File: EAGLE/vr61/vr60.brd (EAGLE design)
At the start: 283 x 93 mm, 222 parts, among them IC1 MC74VHC1G50, IC2 REG1117, J6 MICROMOD-2222-C

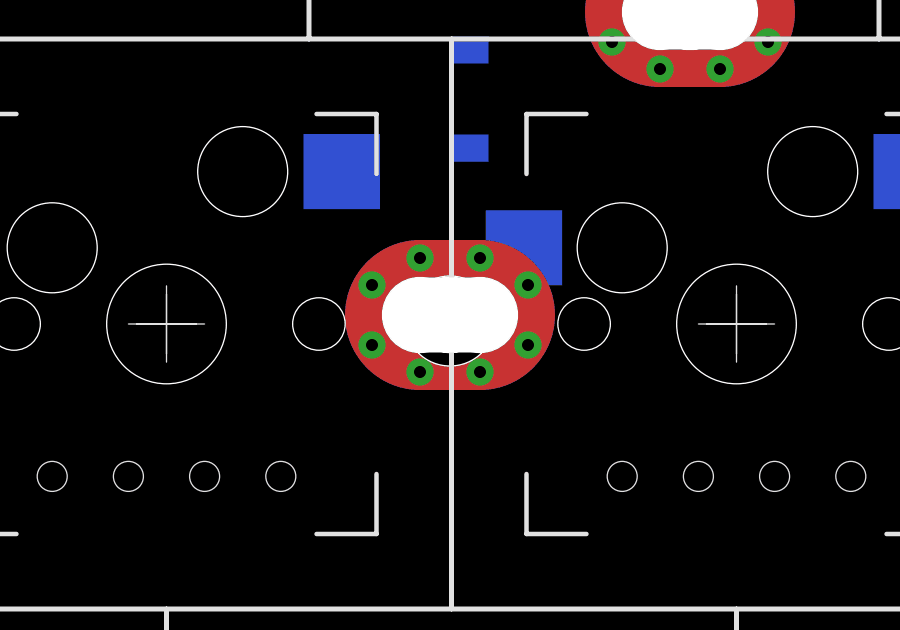
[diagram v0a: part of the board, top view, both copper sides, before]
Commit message: .
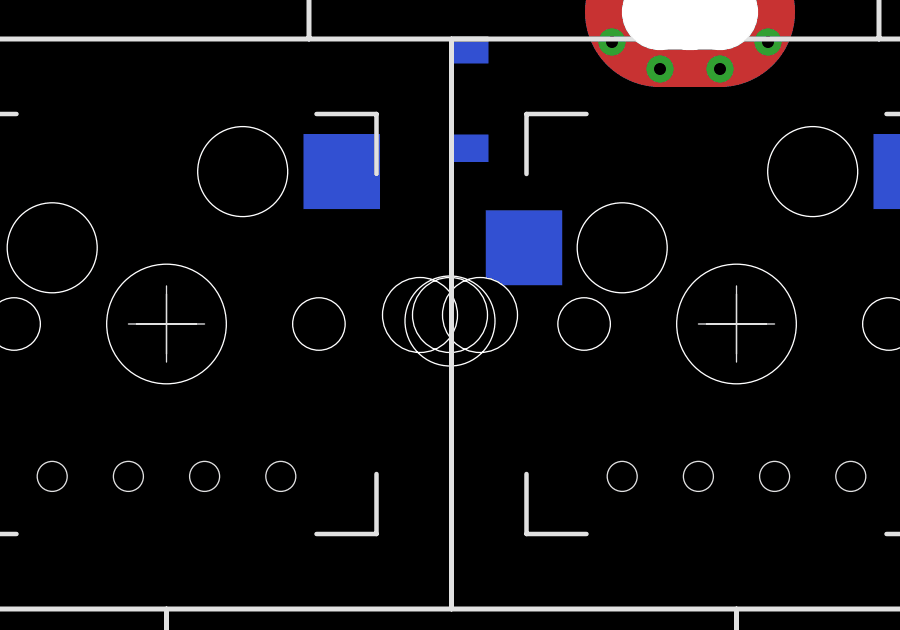
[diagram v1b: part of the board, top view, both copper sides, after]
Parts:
- removed U$9: MOUNTING-HOLE-WIDE, ts_keyboards:MOUNTING-HOLE-WIDE
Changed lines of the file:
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@@
 <drawing>
 <settings>
-<setting alwaysvectorfont="no"/>
+<setting alwaysvectorfont="yes"/>
 <setting verticaltext="up"/>
 </settings>
@@
 <wire x1="22.7" y1="87" x2="22.7" y2="94" width="0.01" layer="49" style="shortdash"/>
 <circle x="29.15" y="46.6" radius="2.5" width="0.01" layer="49"/>
+<hole x="129.2" y="47.8" drill="2.5"/>
+<hole x="127.2" y="47.8" drill="2.5"/>
 </plain>
 <attributes>
@@
 </element>
 <element name="U$8" library="ts_keyboards" package="MOUNTING-HOLE-VWIDE" value="MOUNTING-HOLE-VWIDE" x="282.5" y="38.3" locked="yes" smashed="yes"/>
-<element name="U$9" library="ts_keyboards" package="MOUNTING-HOLE-WIDE" value="MOUNTING-HOLE-WIDE" x="128.2" y="47.8" locked="yes" smashed="yes"/>
 <element name="U$10" library="ts_keyboards" package="MOUNTING-HOLE-WIDE" value="MOUNTING-HOLE-WIDE" x="74.2" y="16.9" locked="yes" smashed="yes"/>
 <element name="U$12" library="ts_keyboards" package="MOUNTING-HOLE-WIDE" value="MOUNTING-HOLE-WIDE" x="190.5" y="9.6" locked="yes" smashed="yes"/>
